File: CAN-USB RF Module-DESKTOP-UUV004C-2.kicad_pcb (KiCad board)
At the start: 2 copper layers, 59.7 x 25.4 mm, 54 parts, among them IC1 ESDALC6V1W5, J1 0022232031, J2 USB_B_Micro, J3 Conn_Coaxial, J4 Conn_01x06_Pin, SW1 RESET, SW2 BOOT0, U2 TLV2217-33KVURG3, U3 SX1280IMLTRT, U4 MCP2542WFDxMF (CAN), U5 FT234XD-R, U6 STM32L442KCU6, Y1 52MHz

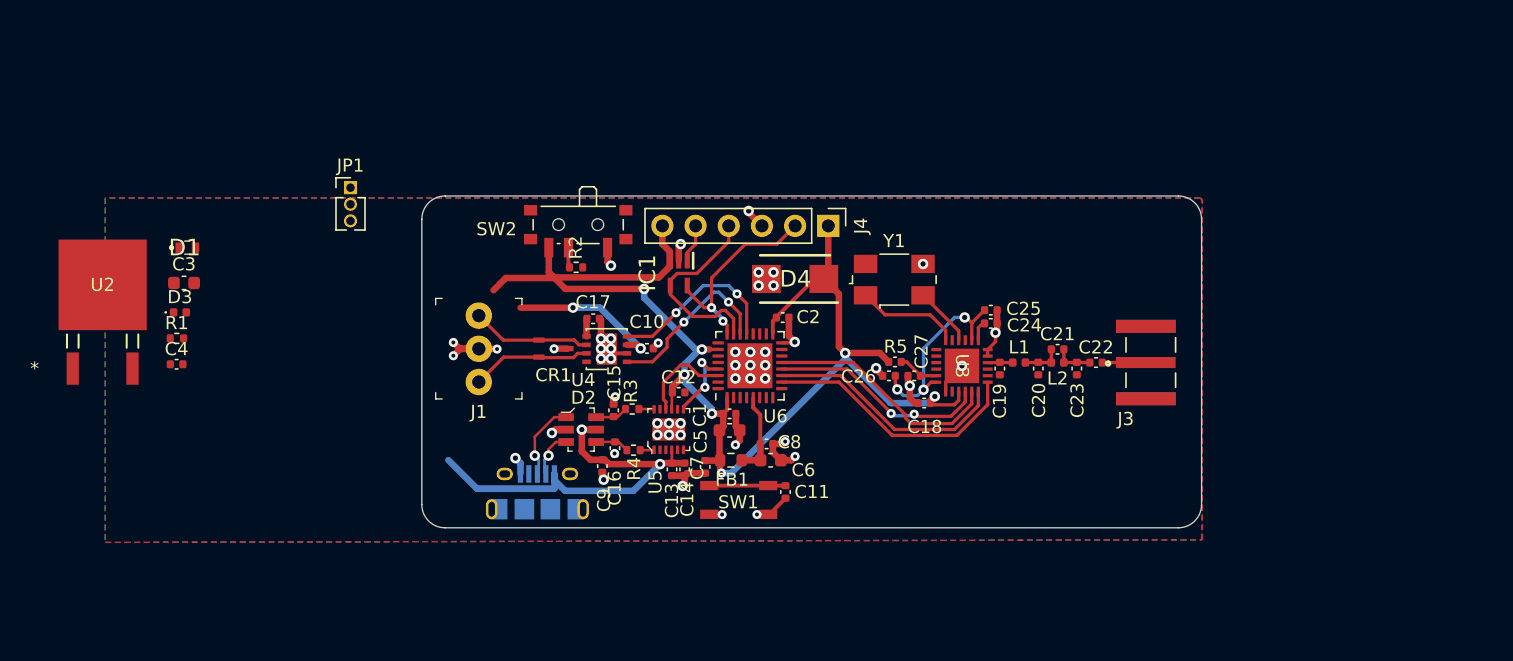
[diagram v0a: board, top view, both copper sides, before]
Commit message: Made minor changes
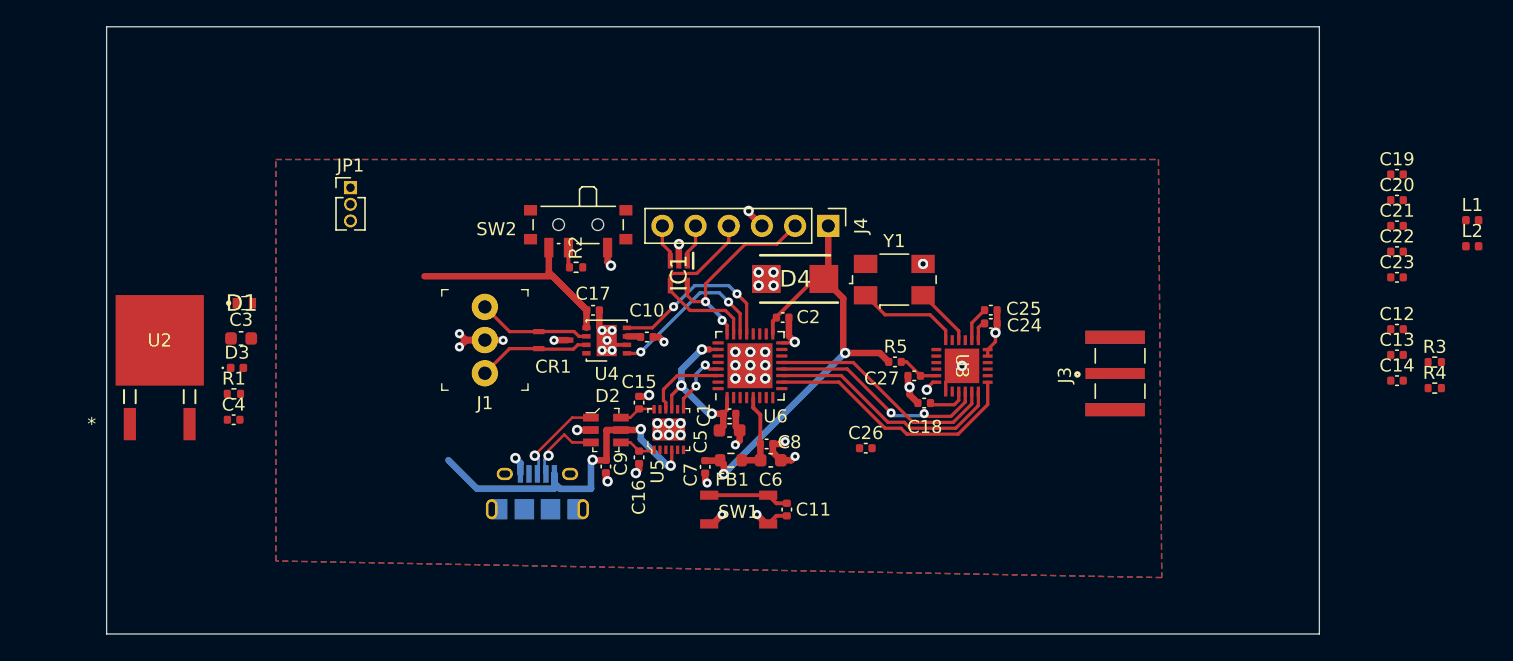
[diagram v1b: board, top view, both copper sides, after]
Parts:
- moved R3 61.5 mm to (187.0, 89.2), turned to 0 degrees
- moved R4 61.5 mm to (187.0, 91.2)
- moved C13 56.2 mm to (184.1, 88.6), turned to 0 degrees
- moved C12 55.2 mm to (184.1, 86.7)
- moved C14 55.0 mm to (184.1, 90.6), turned to 0 degrees
- moved L1 36.4 mm to (189.9, 78.3)
- moved C19 33.8 mm to (184.1, 74.8), turned to 0 degrees
- moved L2 33.0 mm to (189.9, 80.3)
- moved C20 30.3 mm to (184.1, 76.8), turned to 0 degrees
- moved C21 27.6 mm to (184.1, 78.7)
- moved C23 25.5 mm to (184.1, 82.7), turned to 0 degrees
- moved C22 24.6 mm to (184.1, 80.7)
- moved R1 6.09 mm to (95.1, 91.6)
- moved C3 6.09 mm to (95.6, 87.4)
- moved D1 6.09 mm to (95.9, 84.7)
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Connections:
- J3 pad SH1: GND -> (no net)
- J3 pad SH2: GND -> (no net)
- J3 pad SH3: GND -> (no net)
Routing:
- net +3V3: track 100.8 -> 76.5 mm, vias 7 -> 5
- net Net-(U3-DCC_FB): track 15.4 -> 3.73 mm, vias 3 -> 1
- net +5V: track 11.3 -> 1.07 mm, vias 2 -> 0
- net VBUS: track 32.2 -> 27.3 mm, vias 2 -> 3
- net GND: track 48.0 -> 44.4 mm, vias 50 -> 48
- net Net-(J3-In): track 3.33 -> 0.00 mm
- net Net-(C21-Pad2): track 3.06 -> 0.00 mm
- net Net-(C20-Pad1): track 3.06 -> 0.00 mm
- net Net-(U3-RFIO): track 1.95 -> 0.00 mm
- net /USB Interface/USB_D-: track 7.37 -> 8.86 mm
- net /UART1_USB_RX: track 7.21 -> 6.22 mm
- net /UART1_USB_TX: track 5.90 -> 5.19 mm
- net /CAN_TX: track 13.5 -> 12.8 mm
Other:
- board size 59.7 x 25.4 mm -> 92.8 x 46.5 mm
